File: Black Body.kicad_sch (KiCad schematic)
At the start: 28 parts, among them IC2 MCP96L00T-E_MX, J1 53307-2471, J2 Conn_01x02, J3 Conn_01x03, J4 Conn_02x08_Top_Bottom

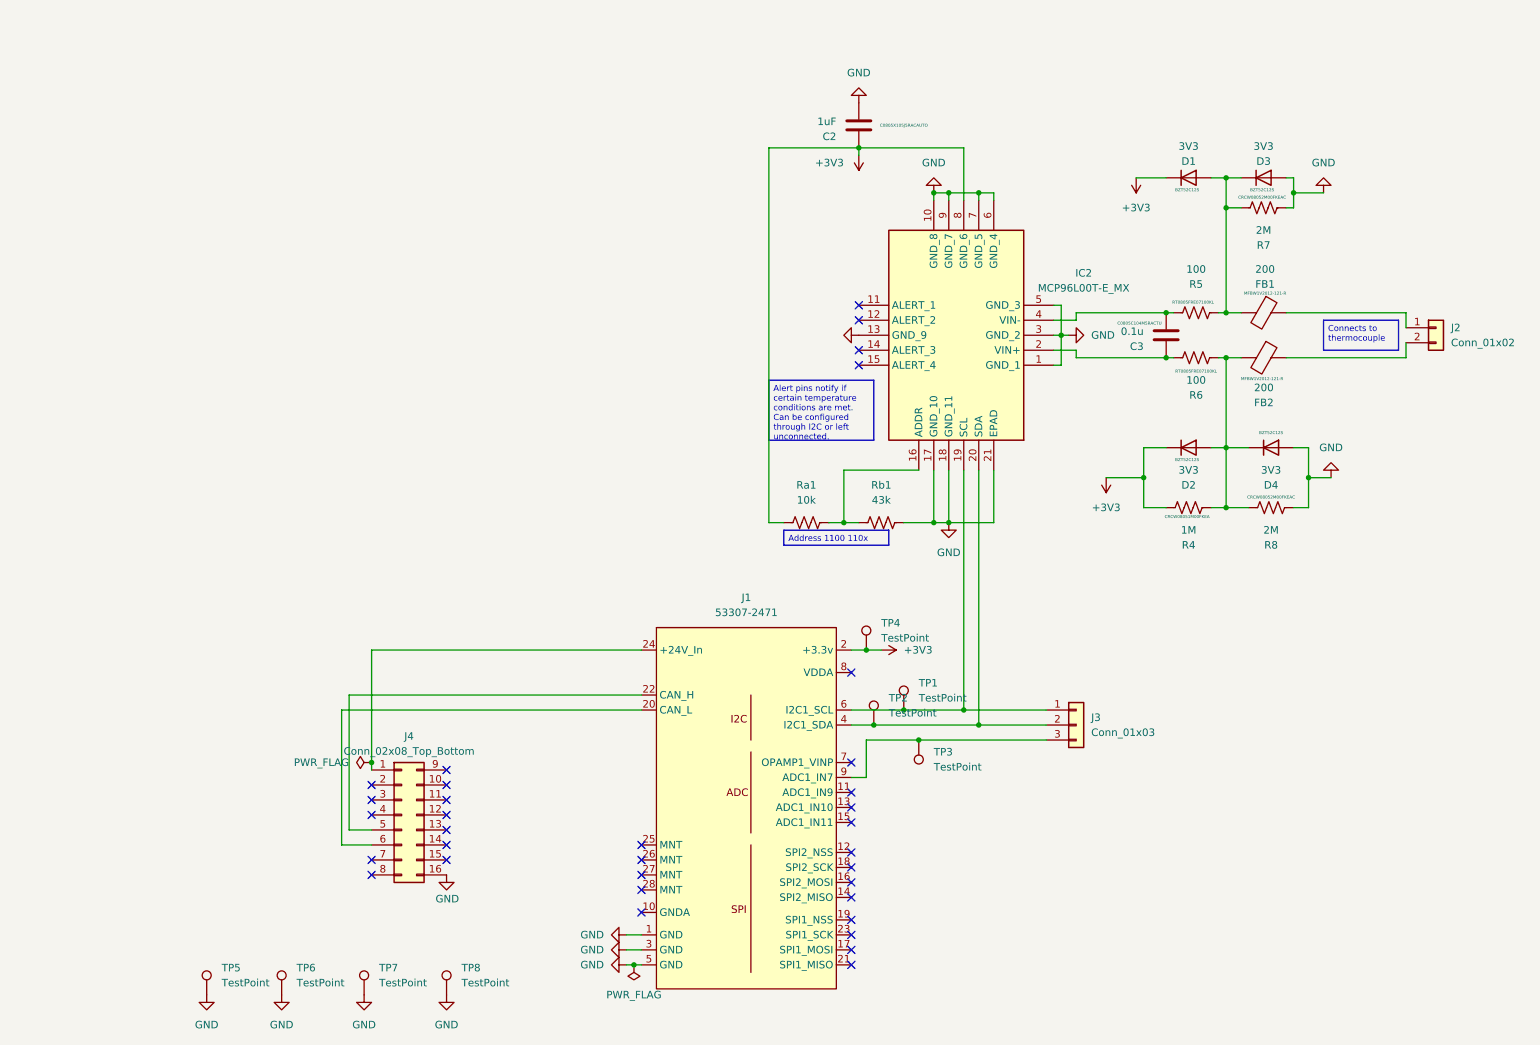
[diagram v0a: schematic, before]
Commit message: Updated Layout
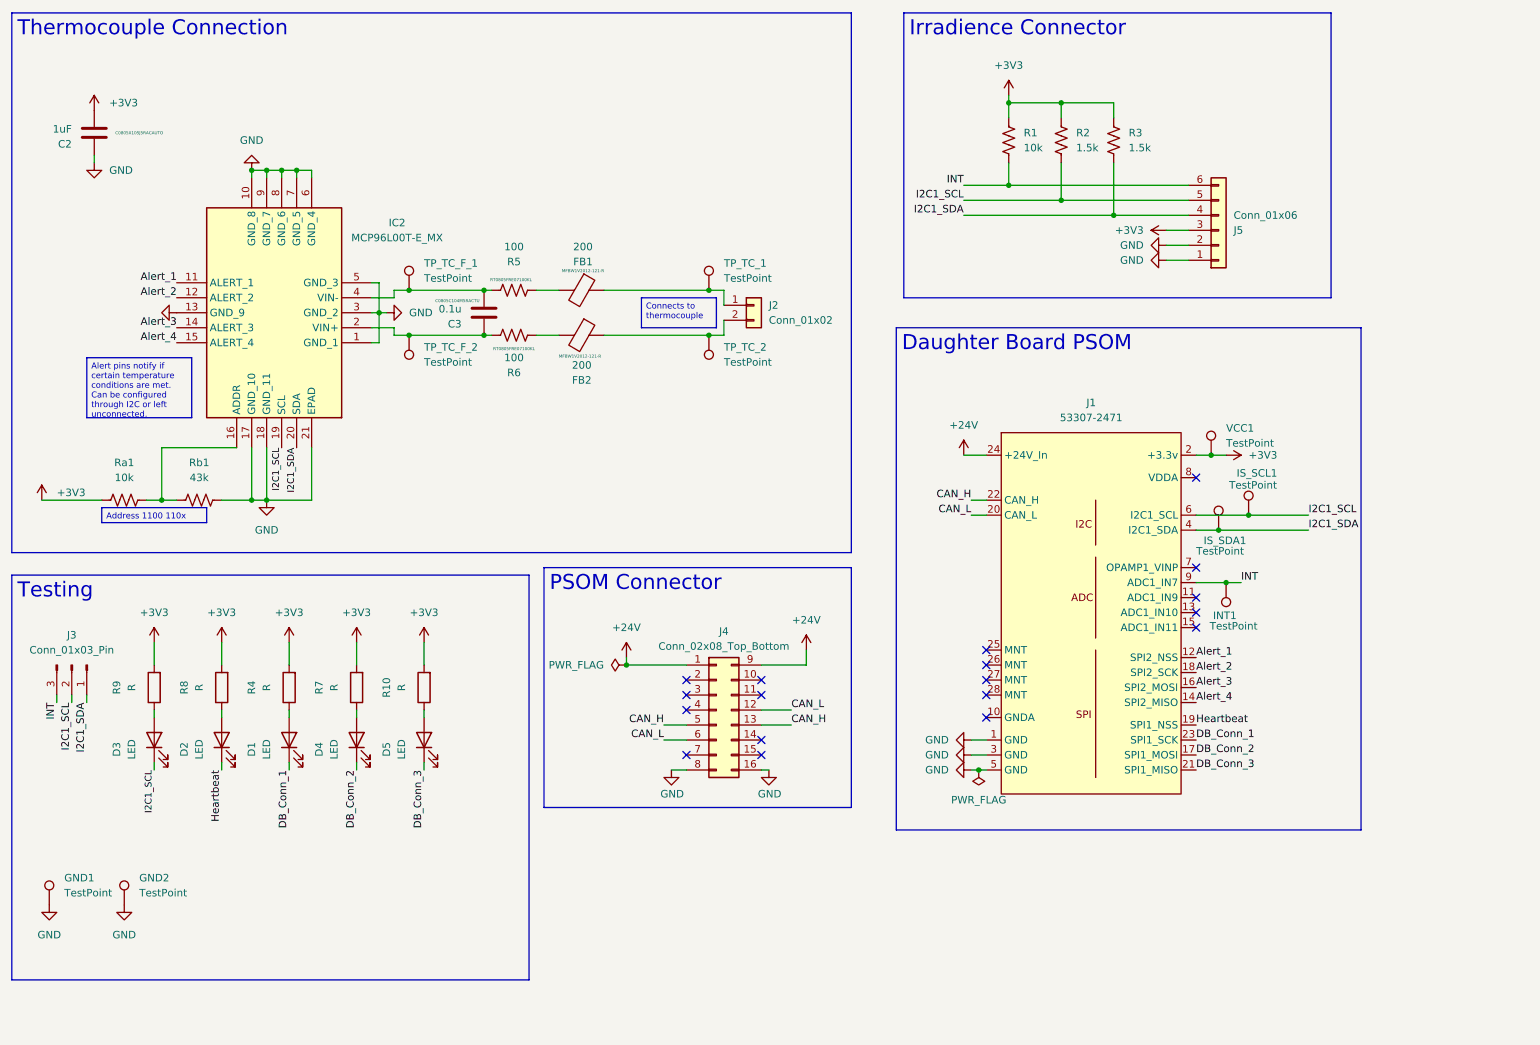
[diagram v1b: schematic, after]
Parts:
- removed D1, D2, D3, D4: 3V3, Diode_SMD:D_0603_1608Metric_Pad1.05x0.95mm_HandSolder, symbol Device:D
- removed J3: Conn_01x03, Connector_Molex:Molex_Nano-Fit_105313-xx03_1x03_P2.50mm_Horizontal, symbol Connector_Generic:Conn_01x03
- removed R4: 1M, Resistor_SMD:R_0603_1608Metric_Pad0.98x0.95mm_HandSolder, symbol Device:R_US
- removed R7, R8: 2M, Resistor_SMD:R_0603_1608Metric_Pad0.98x0.95mm_HandSolder, symbol Device:R_US
- removed TP7, TP8: TestPoint, Connector_PinHeader_2.54mm:PinHeader_1x01_P2.54mm_Vertical, symbol Connector:TestPoint
- added D1, D2, D3, D4, D5: LED, LED_SMD:LED_0603_1608Metric_Pad1.05x0.95mm_HandSolder, symbol Device:LED
- added J3: Conn_01x03_Pin, Connector_Molex:Molex_Nano-Fit_105313-xx03_1x03_P2.50mm_Horizontal, symbol Connector:Conn_01x03_Pin
- added J5: Conn_01x06, Connector_Molex:Molex_Nano-Fit_105313-xx06_1x06_P2.50mm_Horizontal, symbol Connector_Generic:Conn_01x06
- added R1: 10k, Resistor_SMD:R_0805_2012Metric, symbol Device:R_US
- added R10, R4, R7, R8, R9: R, Resistor_SMD:R_0603_1608Metric_Pad0.98x0.95mm_HandSolder, symbol Device:R
- added R2, R3: 1.5k, Resistor_SMD:R_0805_2012Metric, symbol Device:R_US
- added TP_TC_1, TP_TC_2, TP_TC_F_1, TP_TC_F_2: TestPoint, Connector_PinHeader_2.54mm:PinHeader_1x01_P2.54mm_Vertical, symbol Connector:TestPoint
- J4: footprint MX150:CONN_SD-75900-001_2X08_MOL -> Blackbody Footprint:CONN_SD-75900-001_2X08_MOL
- renumbered TP5 to GND1, TP6 to GND2, TP3 to INT1, TP1 to IS_SCL1, TP2 to IS_SDA1, TP4 to VCC1
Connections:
- net +3V3: now also C2.2, J5.3 (Pin_3), R1.1, R10.2, R2.1, R3.1, R4.2, R7.2, R8.2, R9.2; no longer C2.1, IC2.8 (GND_6)
- net GND: now also C2.1, IC2.8 (GND_6), J4.8 (Pin_8), J5.1 (Pin_1), J5.2 (Pin_2); no longer C2.2
- net at FB1.1, J2.1 (Pin_1): now also TP_TC_1.1
- net at C3.1, IC2.2 (VIN+), R6.1: now also TP_TC_F_2.1
- net at C3.2, IC2.4 (VIN-), R5.1: now also TP_TC_F_1.1
- net I2C1_SCL: now reaches IC2.19 (SCL), IS_SCL1.1, J1.6 (I2C1_SCL)
- net I2C1_SCL: now also D3.1 (K), J3.2 (Pin_2), J5.5 (Pin_5), R2.2
- net I2C1_SDA: now reaches IC2.20 (SDA), IS_SDA1.1, J1.4 (I2C1_SDA)
- net I2C1_SDA: now also J3.1 (Pin_1), J5.4 (Pin_4), R3.2
- net INT: now reaches INT1.1, J1.9 (ADC1_IN7)
- net INT: now also J3.3 (Pin_3), J5.6 (Pin_6), R1.2
- net at FB2.1, J2.2 (Pin_2): now also TP_TC_2.1
- net Alert_1: now reaches IC2.11 (ALERT_1)
- net Alert_1: now also J1.12 (SPI2_NSS)
- net Alert_2: now reaches IC2.12 (ALERT_2)
- net Alert_2: now also J1.18 (SPI2_SCK)
- net Alert_3: now reaches IC2.14 (ALERT_3)
- net Alert_3: now also J1.16 (SPI2_MOSI)
- net Alert_4: now reaches IC2.15 (ALERT_4)
- net Alert_4: now also J1.14 (SPI2_MISO)
- net DB_Conn_2: now reaches J1.17 (SPI1_MOSI)
- net DB_Conn_2: now also D4.1 (K)
- net Heartbeat: now reaches J1.19 (SPI1_NSS)
- net Heartbeat: now also D2.1 (K)
- net CAN_L: now reaches J1.20 (CAN_L), J4.6 (Pin_6)
- net CAN_L: now also J4.12 (Pin_12)
- net DB_Conn_3: now reaches J1.21 (SPI1_MISO)
- net DB_Conn_3: now also D5.1 (K)
- net CAN_H: now reaches J1.22 (CAN_H), J4.5 (Pin_5)
- net CAN_H: now also J4.13 (Pin_13)
- net DB_Conn_1: now reaches J1.23 (SPI1_SCK)
- net DB_Conn_1: now also D1.1 (K)
- net +24V: now reaches J1.24 (+24V_In), J4.1 (Pin_1)
- net +24V: now also J4.9 (Pin_9)
- new net: D1.2 (A), R4.1
- new net: D2.2 (A), R8.1
- new net: D4.2 (A), R7.1
- new net: D5.2 (A), R10.1
- new net: D3.2 (A), R9.1
- no-connect marks 34 -> 18
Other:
- moved on the sheet: C2, C3, FB1, FB2, GND1, GND2, IC2, INT1, IS_SCL1, IS_SDA1, J1, J2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
